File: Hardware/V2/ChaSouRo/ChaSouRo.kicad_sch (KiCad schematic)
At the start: 41 parts, among them J3 Conn_ST_STDC14, U1 STM32G431CBUx, Y1 Crystal_GND24_Small

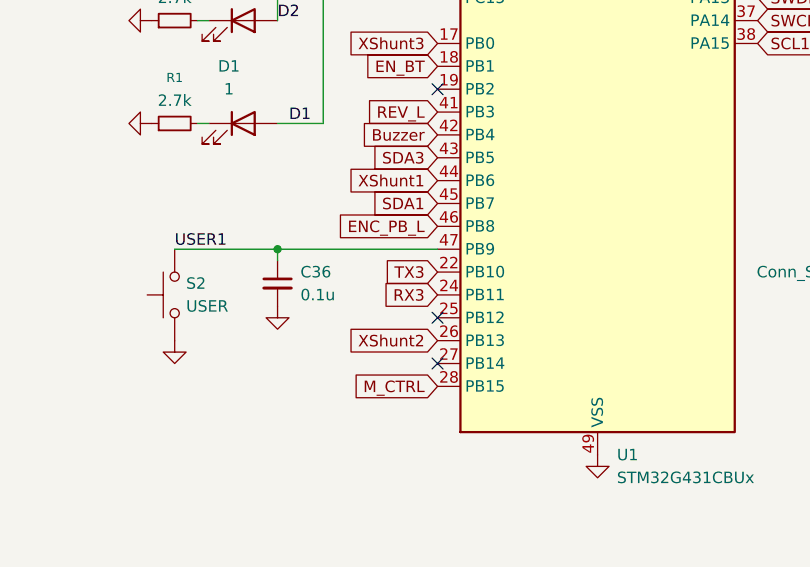
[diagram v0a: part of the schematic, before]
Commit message: modif V2 PCB
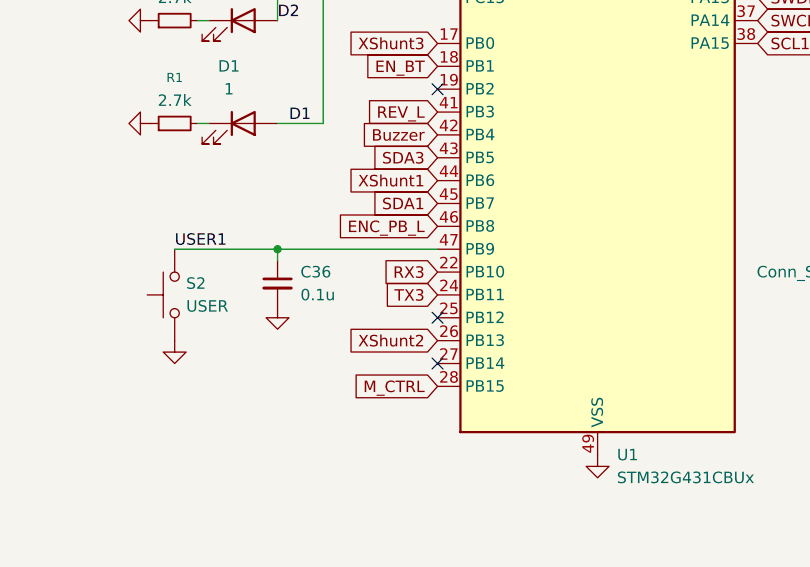
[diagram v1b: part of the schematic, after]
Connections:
- net RX3: now also U1.22 (PB10); no longer U1.24 (PB11)
- net TX3: now also U1.24 (PB11); no longer U1.22 (PB10)
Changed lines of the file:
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@@
+		)
+	)
+	(global_label "ENC_PB_L"
+		(shape input)
+		(at 195.58 113.03 180)
+		(fields_autoplaced yes)
+		(effects
+			(font
+				(size 1.27 1.27)
+			)
+			(justify right)
+		)
+		(property "Intersheetrefs" "${INTERSHEET_REFS}"
+			(at 183.342 113.03 0)
+			(effects
+				(font
+					(size 1.27 1.27)
+				)
+				(justify right)
+				(hide yes)
+			)
+		)
+	)
+	(global_label "LED_STATE"
+		(shape input)
+		(at 231.14 72.39 0)
+		(fields_autoplaced yes)
+		(effects
+			(font
+				(size 1.27 1.27)
+			)
+			(justify left)
+		)
+		(property "Intersheetrefs" "${INTERSHEET_REFS}"
+			(at 243.9222 72.39 0)
+			(effects
+				(font
+					(size 1.27 1.27)
+				)
+				(justify left)
+				(hide yes)
+			)
+		)
+	)
+	(global_label "FWD_L"
+		(shape input)
+		(at 231.14 67.31 0)
+		(fields_autoplaced yes)
+		(effects
+			(font
+				(size 1.27 1.27)
+			)
+			(justify left)
+		)
+		(property "Intersheetrefs" "${INTERSHEET_REFS}"
+			(at 239.9309 67.31 0)
+			(effects
+				(font
+					(size 1.27 1.27)
+				)
+				(justify left)
+				(hide yes)
+			)
+		)
+	)
+	(global_label "REV_L"
+		(shape input)
+		(at 58.42 67.31 180)
+		(fields_autoplaced yes)
+		(effects
+			(font
+				(size 1.27 1.27)
+			)
+			(justify right)
+		)
+		(property "Intersheetrefs" "${INTERSHEET_REFS}"
+			(at 49.9315 67.31 0)
+			(effects
+				(font
+					(size 1.27 1.27)
+				)
+				(justify right)
+				(hide yes)
+			)
+		)
+	)
+	(global_label "TX2"
+		(shape input)
+		(at 231.14 59.69 0)
+		(fields_autoplaced yes)
+		(effects
+			(font
+				(size 1.27 1.27)
+			)
+			(justify left)
+		)
+		(property "Intersheetrefs" "${INTERSHEET_REFS}"
+			(at 237.5118 59.69 0)
+			(effects
+				(font
+					(size 1.27 1.27)
+				)
+				(justify left)
+				(hide yes)
+			)
+		)
+	)
+	(global_label "REV_R"
+		(shape input)
+		(at 87.63 67.31 0)
+		(fields_autoplaced yes)
+		(effects
+			(font
+				(size 1.27 1.27)
+			)
+			(justify left)
+		)
+		(property "Intersheetrefs" "${INTERSHEET_REFS}"
+			(at 96.3604 67.31 0)
+			(effects
+				(font
+					(size 1.27 1.27)
+				)
+				(justify left)
+				(hide yes)
+			)
+		)
+	)
+	(global_label "SDA3"
+		(shape input)
+		(at 49.53 128.27 180)
+		(fields_autoplaced yes)
+		(effects
+			(font
+				(size 1.27 1.27)
+				(thickness 0.1588)
+			)
+			(justify right)
+		)
+		(property "Intersheetrefs" "${INTERSHEET_REFS}"
+			(at 41.2912 128.27 0)
+			(effects
+				(font
+					(size 1.27 1.27)
+				)
+				(justify right)
+				(hide yes)
+			)
+		)
+	)
+	(global_label "SCL3"
+		(shape input)
+		(at 231.14 74.93 0)
+		(fields_autoplaced yes)
+		(effects
+			(font
+				(size 1.27 1.27)
+				(thickness 0.1588)
+			)
+			(justify left)
+		)
+		(property "Intersheetrefs" "${INTERSHEET_REFS}"
+			(at 239.3183 74.93 0)
+			(effects
+				(font
+					(size 1.27 1.27)
+				)
+				(justify left)
+				(hide yes)
+			)
 		)
 	)
 	(global_label "TX3"
 		(shape input)
-		(at 195.58 118.11 180)
-		(fields_autoplaced yes)
-		(effects
-			(font
-				(size 1.27 1.27)
-				(thickness 0.1588)
-			)
-			(justify right)
-		)
-		(property "Intersheetrefs" "${INTERSHEET_REFS}"
-			(at 188.7322 118.11 0)
-			(effects
-				(font
-					(size 1.27 1.27)
-				)
-				(justify right)
-				(hide yes)
-			)
-		)
-	)
-	(global_label "ENC_PB_L"
-		(shape input)
-		(at 195.58 113.03 180)
-		(fields_autoplaced yes)
-		(effects
-			(font
-				(size 1.27 1.27)
-			)
-			(justify right)
-		)
-		(property "Intersheetrefs" "${INTERSHEET_REFS}"
-			(at 183.342 113.03 0)
-			(effects
-				(font
-					(size 1.27 1.27)
-				)
-				(justify right)
-				(hide yes)
-			)
-		)
-	)
-	(global_label "LED_STATE"
-		(shape input)
-		(at 231.14 72.39 0)
-		(fields_autoplaced yes)
-		(effects
-			(font
-				(size 1.27 1.27)
-			)
-			(justify left)
-		)
-		(property "Intersheetrefs" "${INTERSHEET_REFS}"
-			(at 243.9222 72.39 0)
-			(effects
-				(font
-					(size 1.27 1.27)
-				)
-				(justify left)
-				(hide yes)
-			)
-		)
-	)
-	(global_label "FWD_L"
-		(shape input)
-		(at 231.14 67.31 0)
-		(fields_autoplaced yes)
-		(effects
-			(font
-				(size 1.27 1.27)
-			)
-			(justify left)
-		)
-		(property "Intersheetrefs" "${INTERSHEET_REFS}"
-			(at 239.9309 67.31 0)
-			(effects
-				(font
-					(size 1.27 1.27)
-				)
-				(justify left)
-				(hide yes)
-			)
-		)
-	)
-	(global_label "REV_L"
-		(shape input)
-		(at 58.42 67.31 180)
-		(fields_autoplaced yes)
-		(effects
-			(font
-				(size 1.27 1.27)
-			)
-			(justify right)
-		)
-		(property "Intersheetrefs" "${INTERSHEET_REFS}"
-			(at 49.9315 67.31 0)
-			(effects
-				(font
-					(size 1.27 1.27)
-				)
-				(justify right)
-				(hide yes)
-			)
-		)
-	)
-	(global_label "TX2"
-		(shape input)
-		(at 231.14 59.69 0)
-		(fields_autoplaced yes)
-		(effects
-			(font
-				(size 1.27 1.27)
-			)
-			(justify left)
-		)
-		(property "Intersheetrefs" "${INTERSHEET_REFS}"
-			(at 237.5118 59.69 0)
-			(effects
-				(font
-					(size 1.27 1.27)
-				)
-				(justify left)
-				(hide yes)
-			)
-		)
-	)
-	(global_label "REV_R"
-		(shape input)
-		(at 87.63 67.31 0)
-		(fields_autoplaced yes)
-		(effects
-			(font
-				(size 1.27 1.27)
-			)
-			(justify left)
-		)
-		(property "Intersheetrefs" "${INTERSHEET_REFS}"
-			(at 96.3604 67.31 0)
-			(effects
-				(font
-					(size 1.27 1.27)
-				)
-				(justify left)
-				(hide yes)
-			)
-		)
-	)
-	(global_label "SDA3"
-		(shape input)
-		(at 49.53 128.27 180)
-		(fields_autoplaced yes)
-		(effects
-			(font
-				(size 1.27 1.27)
-				(thickness 0.1588)
-			)
-			(justify right)
-		)
-		(property "Intersheetrefs" "${INTERSHEET_REFS}"
-			(at 41.2912 128.27 0)
-			(effects
-				(font
-					(size 1.27 1.27)
-				)
-				(justify right)
-				(hide yes)
-			)
-		)
-	)
-	(global_label "SCL3"
-		(shape input)
-		(at 231.14 74.93 0)
-		(fields_autoplaced yes)
-		(effects
-			(font
-				(size 1.27 1.27)
-				(thickness 0.1588)
-			)
-			(justify left)
-		)
-		(property "Intersheetrefs" "${INTERSHEET_REFS}"
-			(at 239.3183 74.93 0)
-			(effects
-				(font
-					(size 1.27 1.27)
-				)
-				(justify left)
-				(hide yes)
-			)
-		)
-	)
-	(global_label "RX3"
-		(shape input)
 		(at 195.58 120.65 180)
 		(fields_autoplaced yes)
@@
 		)
 		(property "Intersheetrefs" "${INTERSHEET_REFS}"
-			(at 188.4298 120.65 0)
+			(at 188.7322 120.65 0)
 			(effects
 				(font
@@
 			(effects
 				(font
+					(size 1.27 1.27)
+				)
+				(justify right)
+				(hide yes)
+			)
+		)
+	)
+	(global_label "RX3"
+		(shape input)
+		(at 195.58 118.11 180)
+		(fields_autoplaced yes)
+		(effects
+			(font
+				(size 1.27 1.27)
+				(thickness 0.1588)
+			)
+			(justify right)
+		)
+		(property "Intersheetrefs" "${INTERSHEET_REFS}"
+			(at 188.4298 118.11 0)
+			(effects
+				(font
